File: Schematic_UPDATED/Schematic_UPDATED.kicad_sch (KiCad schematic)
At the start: 11 parts, among them U1 AD620ANZ, U3 LM324N, U6 ESP32-DevKitC

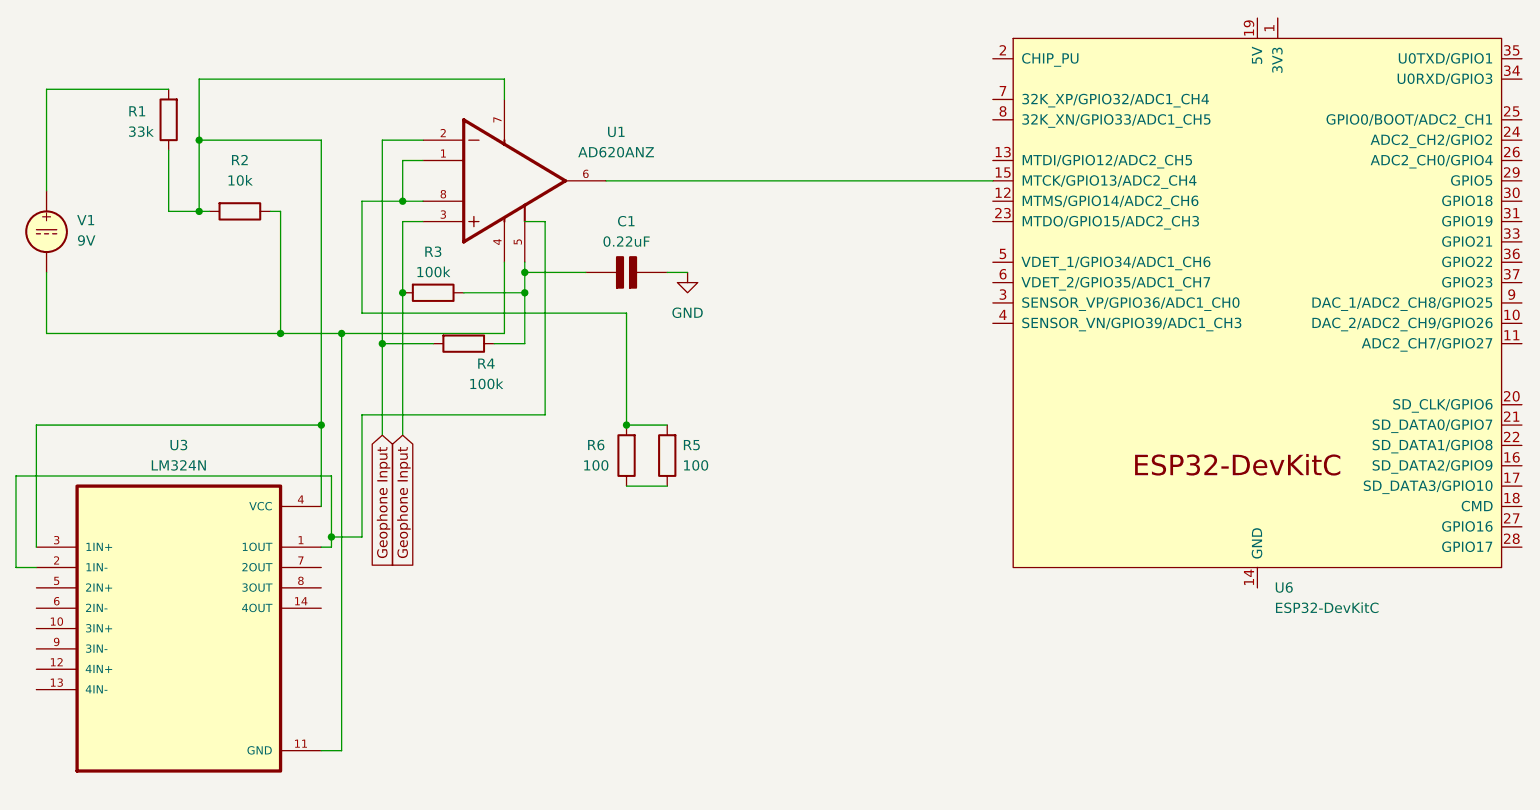
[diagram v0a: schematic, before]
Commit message: Corrections being made
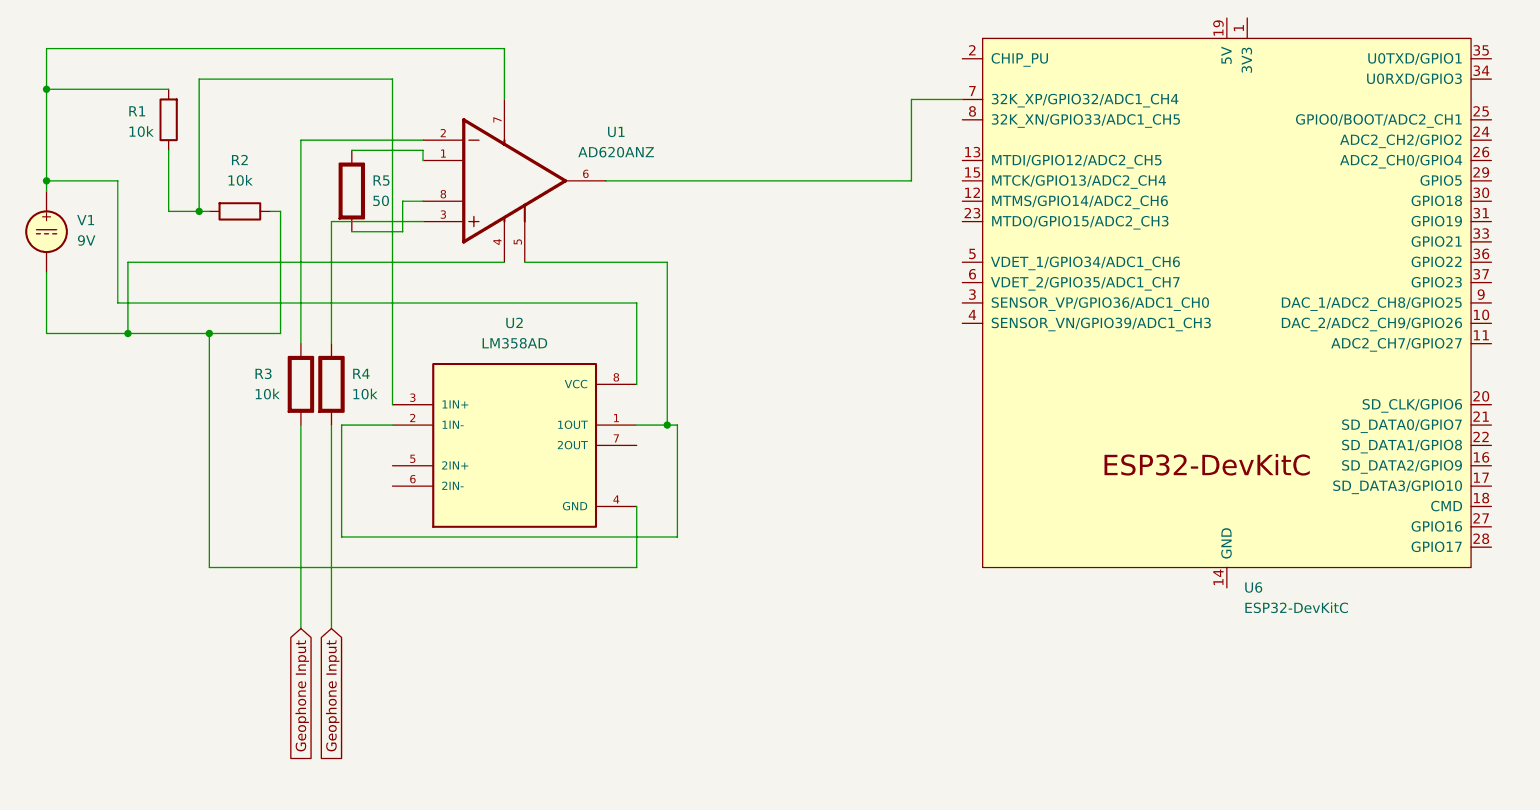
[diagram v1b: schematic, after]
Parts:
- removed C1: 0.22uF, symbol PCM_Elektuur:C
- removed R3, R4: 100k, symbol Device:R
- removed R5, R6: 100, symbol Device:R
- removed U3: LM324N, LM324N:DIP794W45P254L1969H508Q14, symbol LM324N:LM324N
- added R3, R4: 10k, symbol PCM_Elektuur:R
- added R5: 50, symbol PCM_Elektuur:R
- added U2: LM358AD, LM358AD:SOIC127P600X175-8N, symbol LM358AD:LM358AD
- R1: value 33k -> 10k
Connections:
- net Geophone Input: now also R3.2 (-), R4.2 (-); no longer U1.2, U1.3
- net at U1.1: now also R5.1 (+); no longer U1.8
- net at R2.1, U1.4, V1.2: now also U2.4 (GND)
- net at U1.5: now also U2.1 (1OUT), U2.2 (1IN-)
- net at U1.6: now also U6.7 (32K_XP/GPIO32/ADC1_CH4); no longer U6.15 (MTCK/GPIO13/ADC2_CH4)
- net at R1.1, R2.2: now also U2.3 (1IN+); no longer U1.7
- net at R1.2, V1.1: now also U1.7, U2.8 (VCC)
- new net: R3.1 (+), U1.2
- new net: R4.1 (+), U1.3
- new net: R5.2 (-), U1.8
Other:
- moved on the sheet: U6
